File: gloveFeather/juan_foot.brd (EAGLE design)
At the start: 45.7 x 59.4 mm, 9 parts

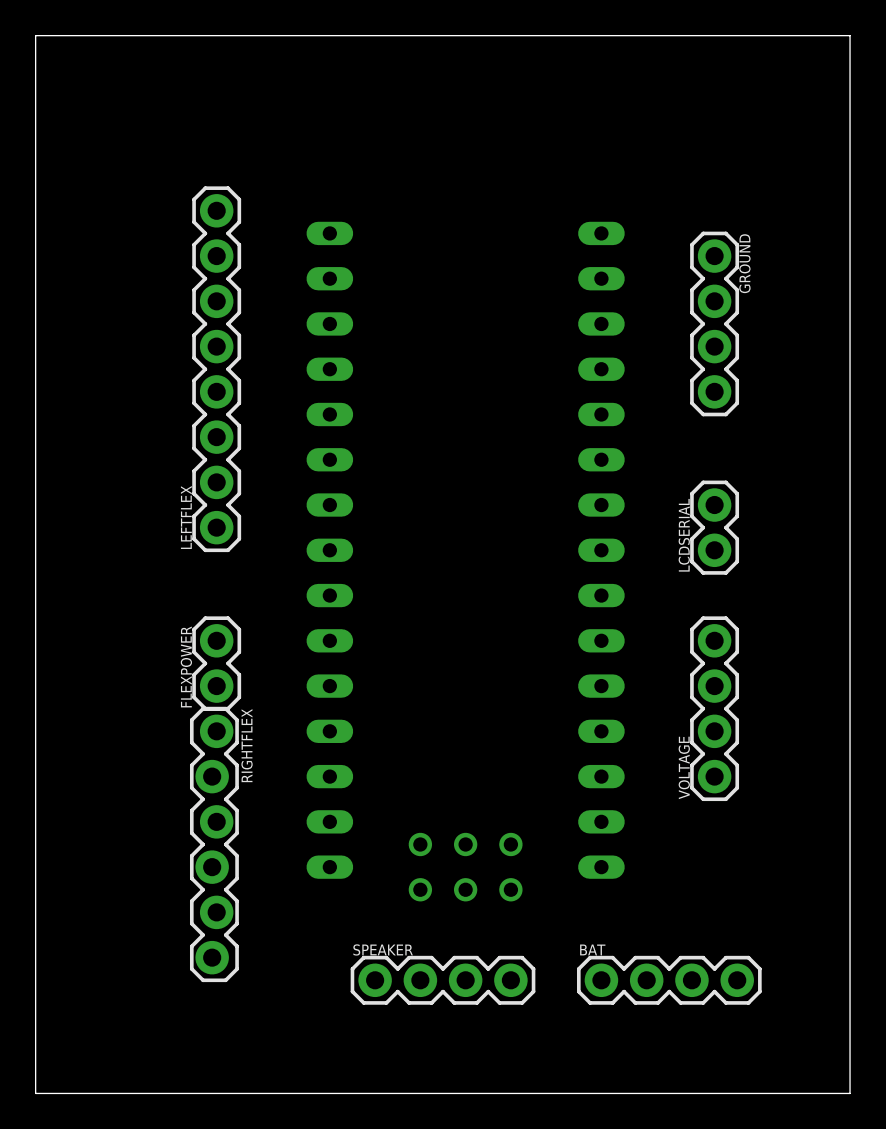
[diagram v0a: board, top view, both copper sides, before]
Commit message: pcb for nano almost ready
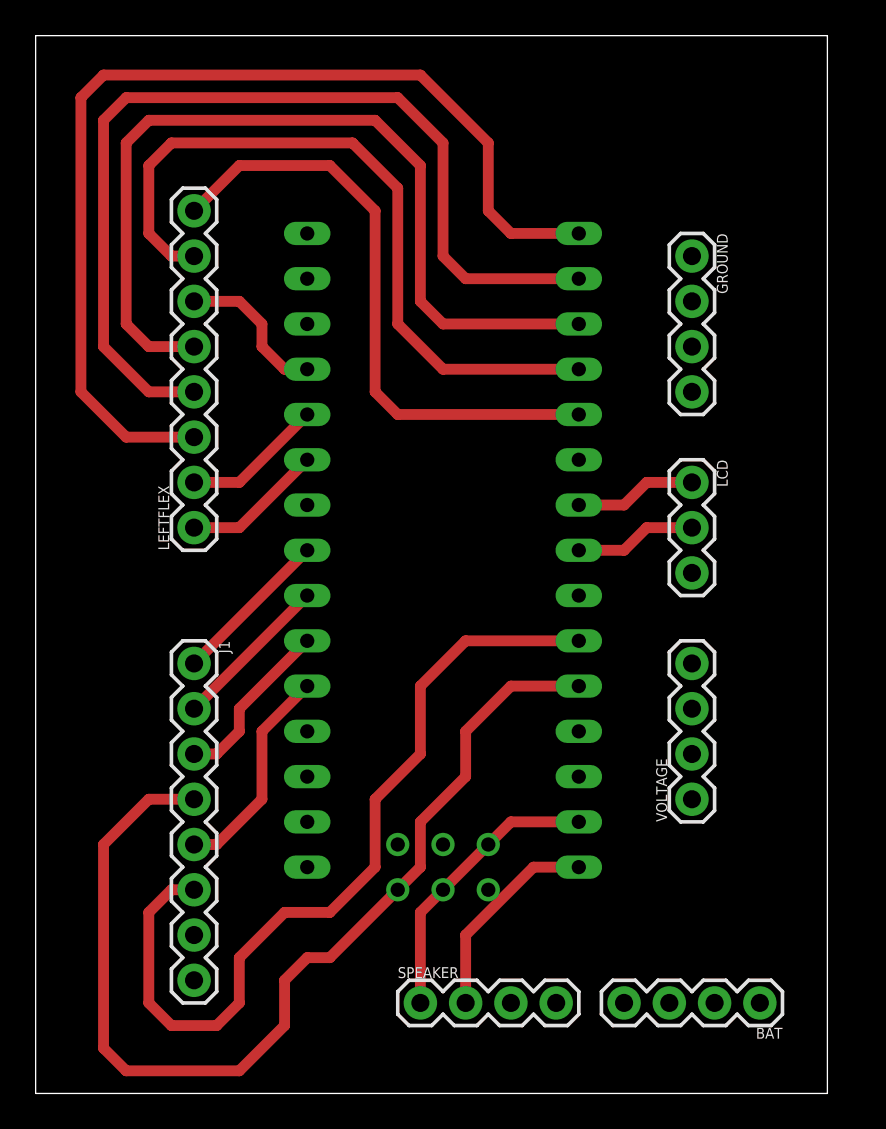
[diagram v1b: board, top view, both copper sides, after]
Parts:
- removed FLEXPOWER, LCDSERIAL: (no value), SparkFun-Connectors:1X02
- removed RIGHTFLEX: (no value), SparkFun-Connectors:1X06_LOCK
- added J1: (no value), SparkFun-Connectors:1X08
- added LCD: (no value), SparkFun-Connectors:1X03
- moved BAT 8.98 mm to (40.6, 5.08), turned to 180 degrees
- moved SPEAKER 2.84 mm to (21.6, 5.08)
- moved VOLTAGE 1.80 mm to (36.8, 16.5)
- moved GROUND 1.27 mm to (36.8, 47.0)
- moved U$1 1.27 mm to (25.4, 21.6)
- moved LEFTFLEX 1.27 mm to (8.89, 31.8)
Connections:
- net 3V: now also J1.8; no longer FLEXPOWER.1, U$1.3.3V
- net GND: now also J1.7, LCD.3; no longer FLEXPOWER.2
- net PINKYFLEX: now also J1.5; no longer RIGHTFLEX.5
- net PINKYSIDE: now also J1.6, U$1.D3; no longer RIGHTFLEX.6, U$1.D2
- net RINGFLEX: now also J1.3; no longer RIGHTFLEX.3
- net RINGSIDE: now also J1.4, U$1.D2; no longer RIGHTFLEX.4, U$1.D3
- net SCL: now also J1.2; no longer RIGHTFLEX.2
- net SDA: now also J1.1; no longer RIGHTFLEX.1
- net SRX: now also LCD.1; no longer LCDSERIAL.2
- net STX: now also LCD.2; no longer LCDSERIAL.1
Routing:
- net INDEXTIP: track 0.00 -> 58.3 mm
- net RINGSIDE: track 0.00 -> 58.2 mm
- net INDEXSIDE: track 0.00 -> 54.0 mm
- net MIDDLETIP: track 0.00 -> 49.6 mm
- net PINKYSIDE: track 0.00 -> 47.7 mm
- net MIDDLESIDE: track 0.00 -> 41.3 mm
- net MIDDLEB: track 0.00 -> 34.4 mm
- net SIN: track 0.00 -> 16.1 mm
- net PINKYFLEX: track 0.00 -> 12.3 mm
- net SOUT: track 0.00 -> 11.7 mm
- net RINGFLEX: track 0.00 -> 9.72 mm
- net SDA: track 0.00 -> 8.98 mm
- net SCL: track 0.00 -> 8.98 mm
- net MIDDLEFLEX: track 0.00 -> 8.67 mm
- net THUMBFLEX: track 0.00 -> 7.93 mm
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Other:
- board size 45.7 x 59.4 mm -> 44.4 x 59.4 mm
